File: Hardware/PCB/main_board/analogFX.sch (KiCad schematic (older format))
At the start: 20 parts, among them Q1 BC547, U1 MCP6002-xSN

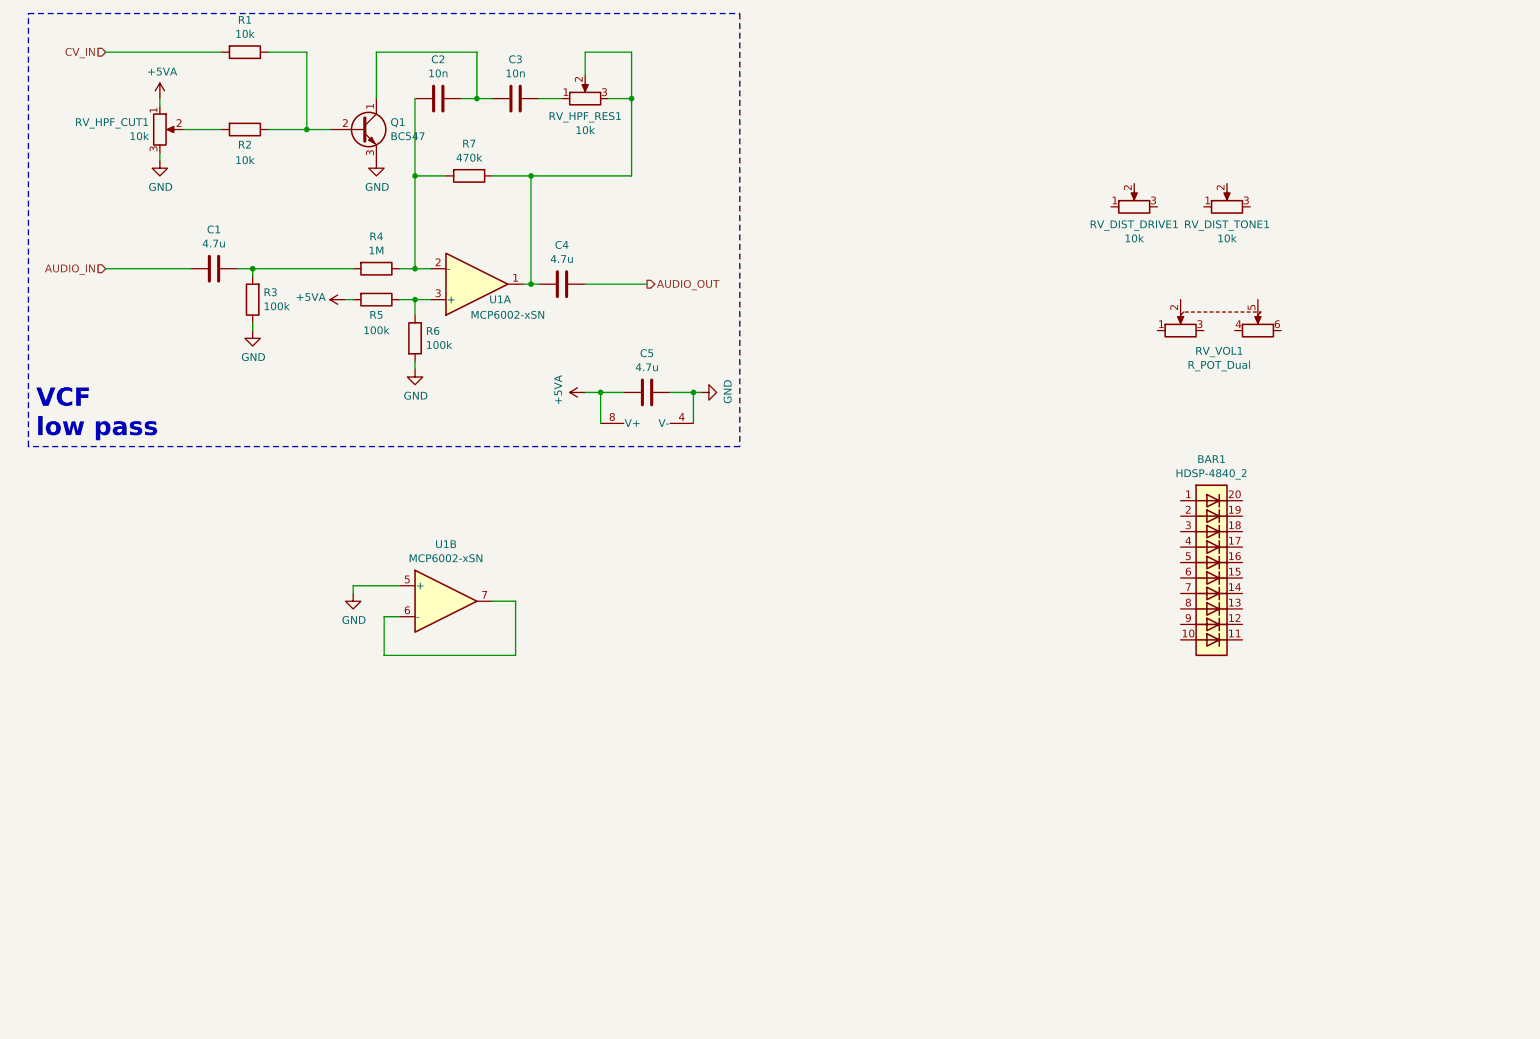
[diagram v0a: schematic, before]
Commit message: Route PWR
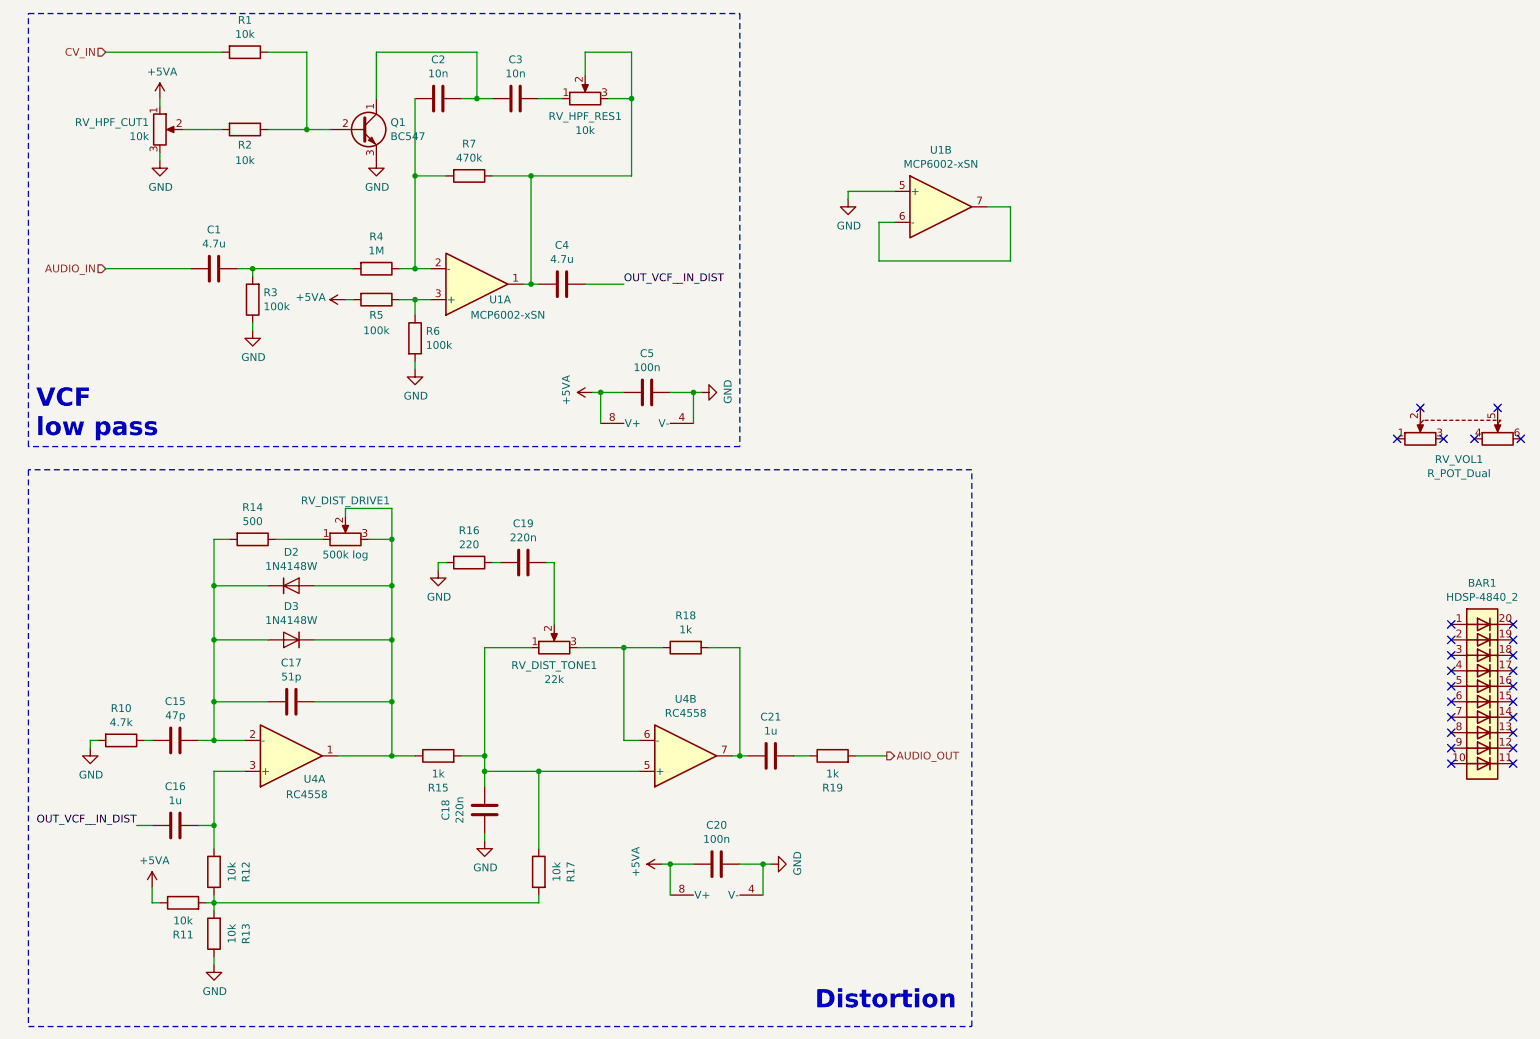
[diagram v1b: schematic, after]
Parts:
- added C15: 47p, Capacitor_SMD:C_0805_2012Metric, symbol Device:C
- added C16, C21: 1u, Capacitor_SMD:C_0805_2012Metric, symbol Device:C
- added C17: 51p, Capacitor_SMD:C_0805_2012Metric, symbol Device:C
- added C18, C19: 220n, Capacitor_SMD:C_0805_2012Metric, symbol Device:C
- added C20: 100n, Capacitor_SMD:C_0805_2012Metric, symbol Device:C
- added D2, D3: 1N4148W, Diode_SMD:D_SOD-123, symbol Diode:1N4148W
- added R10: 4.7k, Resistor_SMD:R_0805_2012Metric, symbol Device:R
- added R11, R12, R13, R17: 10k, Resistor_SMD:R_0805_2012Metric, symbol Device:R
- added R14: 500, Resistor_SMD:R_0805_2012Metric, symbol Device:R
- added R15, R18, R19: 1k, Resistor_SMD:R_0805_2012Metric, symbol Device:R
- added R16: 220, Resistor_SMD:R_0805_2012Metric, symbol Device:R
- added U4: RC4558, Package_SO:SOIC-8_3.9x4.9mm_P1.27mm, symbol Amplifier_Operational:RC4558
- C5: value 4.7u -> 100n
- RV_DIST_DRIVE1: value 10k -> 500k log
- RV_DIST_TONE1: value 10k -> 22k
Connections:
- net +5VA: now also C20.2, R11.1, U4.8 (V+)
- net AUDIO_OUT: now also R19.2; no longer C4.1
- net GND: now also C18.2, C20.1, R10.2, R13.1, R16.2, U4.4 (V-)
- net at RV_DIST_DRIVE1.1: now also R14.1
- net at RV_DIST_DRIVE1.2: now also RV_DIST_DRIVE1.3, C17.1, D2.2 (A), D3.1 (K), R15.1, U4.1
- net at RV_DIST_TONE1.1: now also C18.1, R15.2, R17.1, U4.5 (+)
- net at RV_DIST_TONE1.2: now also C19.1
- net at RV_DIST_TONE1.3: now also R18.1, U4.6 (-)
- new net: C15.1, C17.2, D2.1 (K), D3.2 (A), R14.2, U4.2 (-)
- new net: C16.1, R12.2, U4.3 (+)
- new net: C21.2, R18.2, U4.7
- new net: C15.2, R10.1
- new net: R11.2, R12.1, R13.2, R17.2
- new net: C19.2, R16.1
- new net: C21.1, R19.1
- new net OUT_VCF__IN_DIST: C16.2, C4.1
- no-connect marks 0 -> 26
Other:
- note added: "Distortion"
- moved on the sheet: BAR1, RV_DIST_DRIVE1, RV_DIST_TONE1, RV_VOL1, U1B
